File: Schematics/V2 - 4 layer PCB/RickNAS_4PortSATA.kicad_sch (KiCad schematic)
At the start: 34 parts, among them J1 2227595-1, J10 10076579-002C-TRLF, J2 Conn_01x03, J3 Conn_01x03, J6 POWER, J7 10076579-002C-TRLF, J8 10076579-002C-TRLF, J9 10076579-002C-TRLF, U1 CH32V003FxPx, U2 TLV1117-33

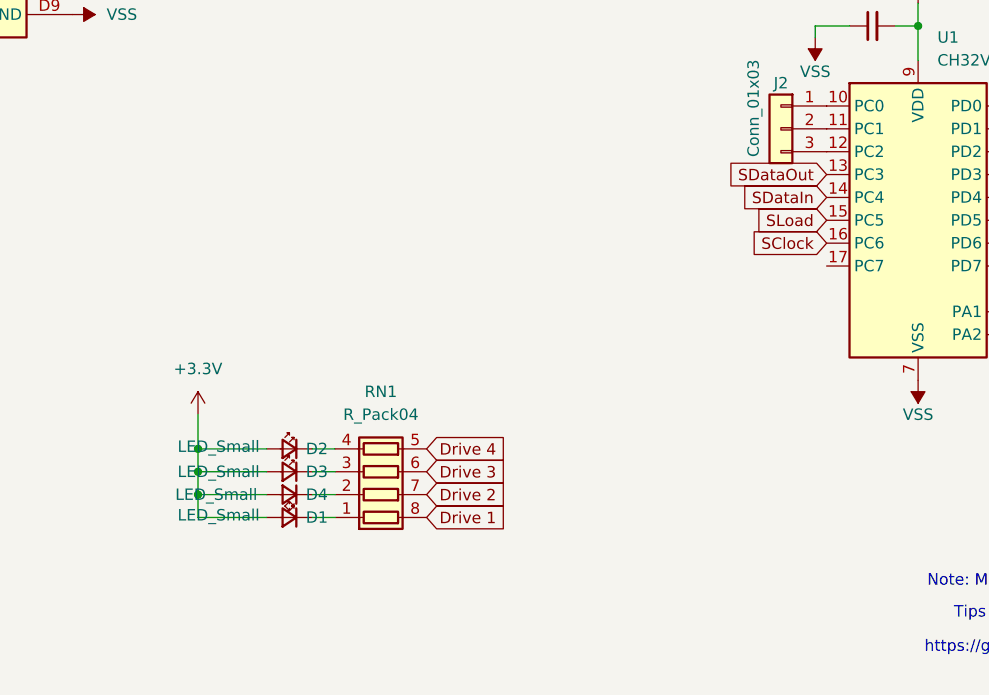
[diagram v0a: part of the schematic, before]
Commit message: ran erc
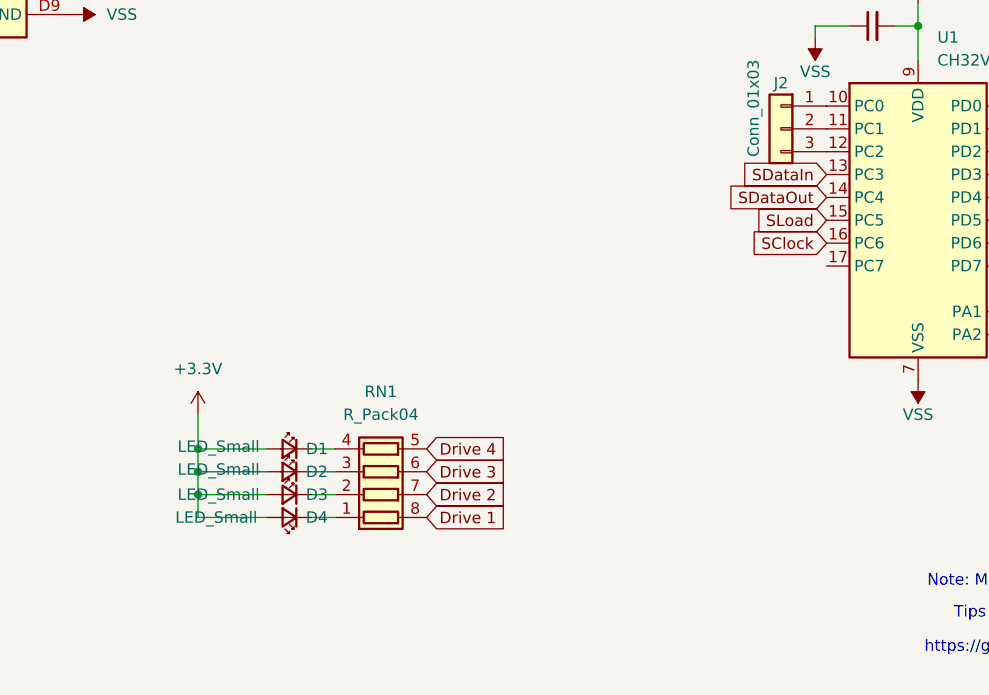
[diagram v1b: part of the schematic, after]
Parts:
- J10, J7, J8, J9: footprint UE_Connector:CONN_10076579-002C-TRLF_AMP -> UE_Connector:91908-291512_SAS_Conn
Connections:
- net SDataIn: now also U1.13 (PC3); no longer U1.14 (PC4)
- net SDataOut: now also U1.14 (PC4); no longer U1.13 (PC3)
- net at D1.1 (K): now also RN1.4 (R4.1); no longer RN1.1 (R1.1)
- net at D4.1 (K): now also RN1.1 (R1.1); no longer RN1.2 (R2.1)
- net at D3.1 (K): now also RN1.2 (R2.1); no longer RN1.3 (R3.1)
- net at D2.1 (K): now also RN1.3 (R3.1); no longer RN1.4 (R4.1)
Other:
- moved on the sheet: D1, D2, D3, D4
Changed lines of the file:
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@@
 	(global_label "SDataOut"
 		(shape input)
-		(at 181.61 125.73 180)
+		(at 181.61 128.27 180)
 		(fields_autoplaced yes)
 		(effects
@@
 		)
 		(property "Intersheetrefs" "${INTERSHEET_REFS}"
-			(at 169.9164 125.73 0)
+			(at 169.9164 128.27 0)
 			(effects
 				(font
@@
 	(global_label "SDataIn"
 		(shape input)
-		(at 181.61 128.27 180)
+		(at 181.61 125.73 180)
 		(fields_autoplaced yes)
 		(effects
@@
 		)
 		(property "Intersheetrefs" "${INTERSHEET_REFS}"
-			(at 171.3678 128.27 0)
+			(at 171.3678 125.73 0)
 			(effects
 				(font
@@
 	(symbol
 		(lib_id "Device:LED_Small")
-		(at 121.92 163.83 0)
+		(at 121.92 156.21 0)
 		(mirror y)
 		(unit 1)
@@
 		(dnp no)
 		(property "Reference" "D1"
-			(at 124.968 163.83 0)
+			(at 124.968 156.21 0)
 			(effects
 				(font
@@
 		)
 		(property "Value" "LED_Small"
-			(at 114.046 163.576 0)
+			(at 114.046 155.956 0)
 			(effects
 				(font
@@
 		)
 		(property "Footprint" "LED_SMD:LED_0805_2012Metric"
-			(at 121.92 163.83 90)
+			(at 121.92 156.21 90)
 			(effects
 				(font
@@
 		)
 		(property "Datasheet" "~"
-			(at 121.92 163.83 90)
+			(at 121.92 156.21 90)
 			(effects
 				(font
@@
 		)
 		(property "Description" "Light emitting diode, small symbol"
-			(at 121.92 163.83 0)
+			(at 121.92 156.21 0)
 			(effects
 				(font
@@
 			)
 		)
-		(property "Footprint" "UE_Connector:CONN_10076579-002C-TRLF_AMP"
+		(property "Footprint" "UE_Connector:91908-291512_SAS_Conn"
 			(at 122.936 73.66 0)
 			(effects
@@
 			)
 		)
-		(property "Footprint" "UE_Connector:CONN_10076579-002C-TRLF_AMP"
+		(property "Footprint" "UE_Connector:91908-291512_SAS_Conn"
 			(at 202.946 33.02 0)
 			(effects
@@
 			)
 		)
-		(property "Footprint" "UE_Connector:CONN_10076579-002C-TRLF_AMP"
+		(property "Footprint" "UE_Connector:91908-291512_SAS_Conn"
 			(at 202.946 73.66 0)
 			(effects
@@
 			)
 		)
-		(property "Footprint" "UE_Connector:CONN_10076579-002C-TRLF_AMP"
+		(property "Footprint" "UE_Connector:91908-291512_SAS_Conn"
 			(at 122.936 33.02 0)
 			(effects
@@
 	(symbol
 		(lib_id "Device:LED_Small")
-		(at 121.92 156.21 0)
+		(at 121.92 158.75 0)
 		(mirror y)
 		(unit 1)
@@
 		(dnp no)
 		(property "Reference" "D2"
-			(at 124.968 156.21 0)
+			(at 124.968 158.75 0)
 			(effects
 				(font
@@
 		)
 		(property "Value" "LED_Small"
-			(at 114.046 155.956 0)
+			(at 114.046 158.496 0)
 			(effects
 				(font
@@
 		)
 		(property "Footprint" "LED_SMD:LED_0805_2012Metric"
-			(at 121.92 156.21 90)
+			(at 121.92 158.75 90)
 			(effects
 				(font
@@
 		)
 		(property "Datasheet" "~"
-			(at 121.92 156.21 90)
+			(at 121.92 158.75 90)
 			(effects
 				(font
@@
 		)
 		(property "Description" "Light emitting diode, small symbol"
-			(at 121.92 156.21 0)
+			(at 121.92 158.75 0)
 			(effects
 				(font
@@
 	(symbol
 		(lib_id "Device:LED_Small")
-		(at 121.92 161.29 180)
+		(at 121.92 163.83 180)
 		(unit 1)
 		(exclude_from_sim no)
@@
 		(dnp no)
 		(property "Reference" "D4"
-			(at 124.968 161.29 0)
+			(at 124.968 163.83 0)
 			(effects
 				(font
@@
 		)
 		(property "Value" "LED_Small"
-			(at 113.792 161.29 0)
+			(at 113.792 163.83 0)
 			(effects
 				(font
@@
 		)
 		(property "Footprint" "LED_SMD:LED_0805_2012Metric"
-			(at 121.92 161.29 90)
+			(at 121.92 163.83 90)
 			(effects
 				(font
@@
 		)
 		(property "Datasheet" "~"
-			(at 121.92 161.29 90)
+			(at 121.92 163.83 90)
 			(effects
 				(font
@@
 		)
 		(property "Description" "Light emitting diode, small symbol"
-			(at 121.92 161.29 0)
+			(at 121.92 163.83 0)
 			(effects
 				(font
@@
 	(symbol
 		(lib_id "Device:LED_Small")
-		(at 121.92 158.75 0)
+		(at 121.92 161.29 0)
 		(mirror y)
 		(unit 1)
@@
 		(dnp no)
 		(property "Reference" "D3"
-			(at 124.968 158.75 0)
+			(at 124.968 161.29 0)
 			(effects
 				(font
@@
 		)
 		(property "Value" "LED_Small"
-			(at 114.046 158.75 0)
+			(at 114.046 161.29 0)
 			(effects
 				(font
@@
 		)
 		(property "Footprint" "LED_SMD:LED_0805_2012Metric"
-			(at 121.92 158.75 90)
+			(at 121.92 161.29 90)
 			(effects
 				(font
@@
 		)
 		(property "Datasheet" "~"
-			(at 121.92 158.75 90)
+			(at 121.92 161.29 90)
 			(effects
 				(font
@@
 		)
 		(property "Description" "Light emitting diode, small symbol"
-			(at 121.92 158.75 0)
+			(at 121.92 161.29 0)
 			(effects
 				(font
